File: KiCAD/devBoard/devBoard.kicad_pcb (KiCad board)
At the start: 2 copper layers, 31.1 x 66 mm, 4 parts, among them J1 Conn_02x14_Counter_Clockwise, J2 ISP_header_Conn_02x05_Odd_Even, J3 ISP_header_Conn_02x05_Odd_Even, J4 ISP_header_Conn_02x05_Odd_Even

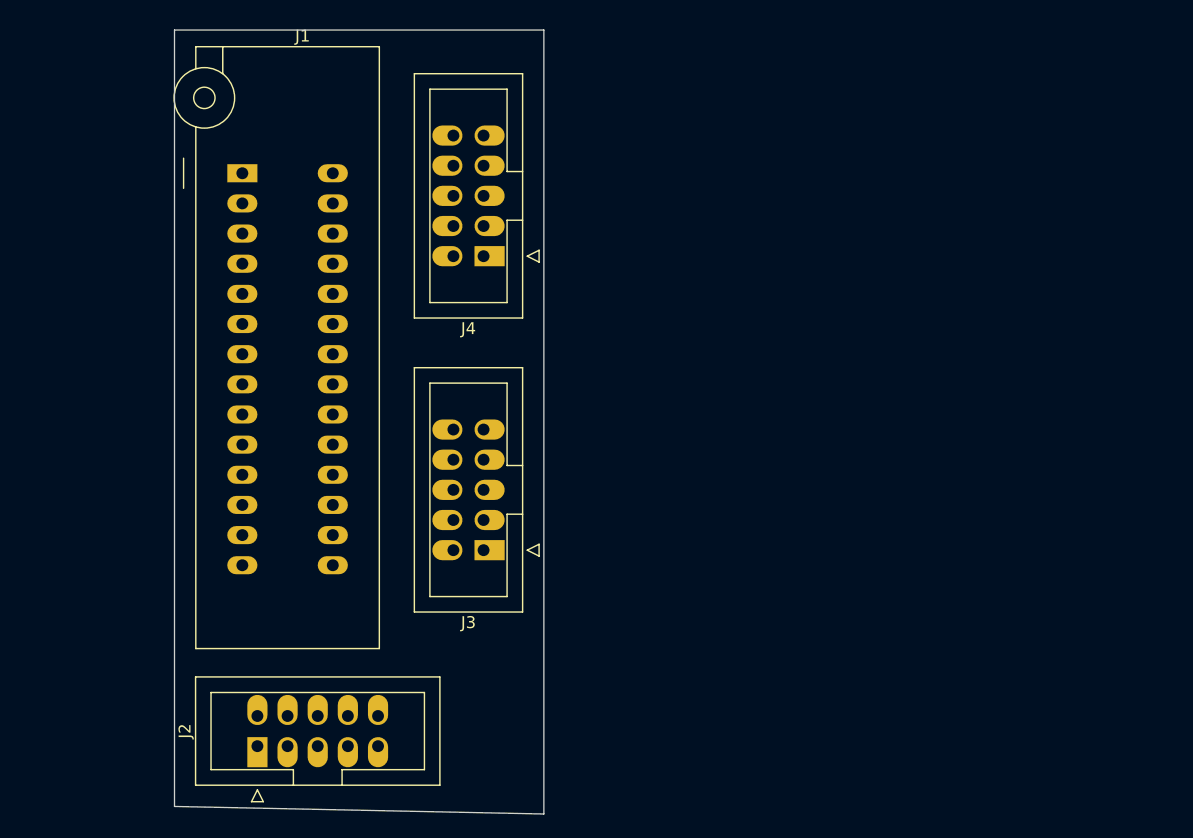
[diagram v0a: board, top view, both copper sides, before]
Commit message: devBoard, gerbers
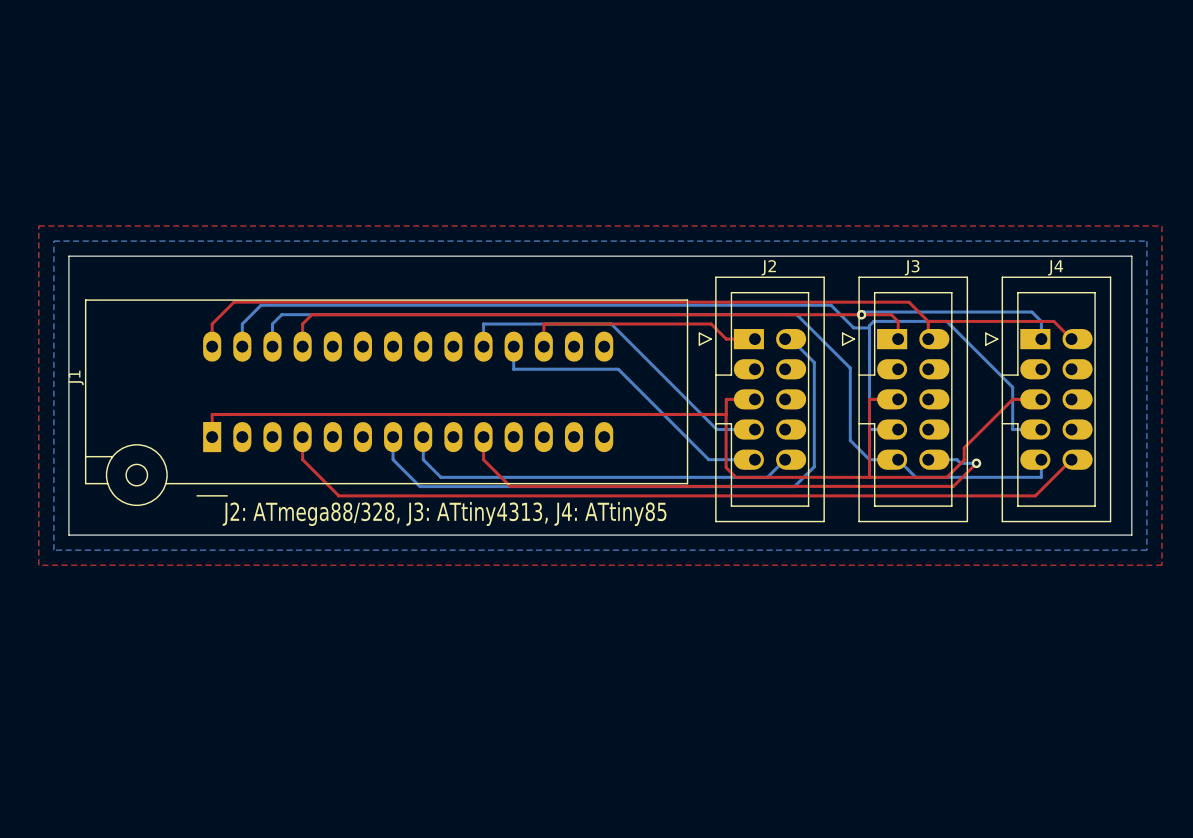
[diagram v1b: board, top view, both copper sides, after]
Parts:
- moved J2 54.2 mm to (188.6, 81.9), turned to 0 degrees
- moved J4 47.5 mm to (212.7, 81.9), turned to 0 degrees
- moved J3 39.2 mm to (200.7, 81.9), turned to 0 degrees
- moved J1 22.4 mm to (142.9, 90.2), turned to 90 degrees
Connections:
- J1 pad 20: 20 -> Net-(J1-Pad20)
- J1 pad 22: 22 -> Net-(J1-Pad22)
- J1 pad 7: 20 -> 7
- J1 pad 8: 22 -> 8
- J2 pad 10: 22 -> 8
- J2 pad 2: 20 -> 7
- J2 pad 8: 22 -> Net-(J2-Pad8)
- J3 pad 8: 10 -> Net-(J3-Pad8)
- J4 pad 8: 4 -> Net-(J4-Pad8)
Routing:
- net 1: track 0.00 -> 92.6 mm
- net 27: track 0.00 -> 87.8 mm
- net 28: track 0.00 -> 79.1 mm
- net 26: track 0.00 -> 77.7 mm
- net 25: track 0.00 -> 71.2 mm, vias 0 -> 1
- net 4: track 0.00 -> 69.2 mm
- net 7: track 0.00 -> 51.1 mm
- net 10: track 0.00 -> 49.3 mm, vias 0 -> 1
- net 8: track 0.00 -> 33.6 mm
- net 19: track 0.00 -> 28.4 mm
- net 18: track 0.00 -> 25.4 mm
- net 17: track 0.00 -> 20.2 mm
- added copper zone on B.Cu, net (none)
- added copper zone on F.Cu, net (none)
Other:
- board size 31.1 x 66 mm -> 89.5 x 23.5 mm
- board text added: "J2: ATmega88/328 J3: ATtiny4313 J4: ATtiny85"
- board text added: "J2: ATmega88/328, J3: ATtiny4313, J4: ATtiny85"
- board text added: "devBoard Design: Jon Sagebrand jonsagebrand@gmail.com"

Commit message: New PCBs
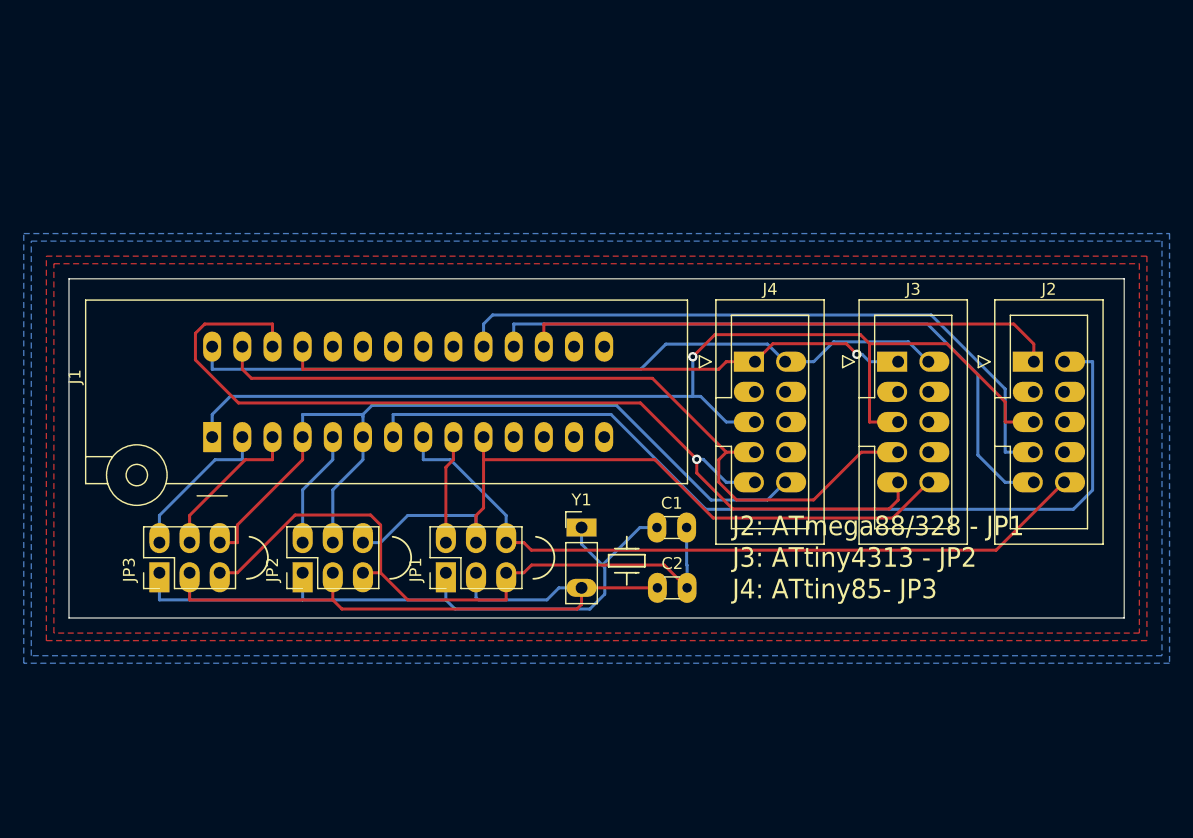
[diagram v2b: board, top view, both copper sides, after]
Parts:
- added C1: 22p, My_Misc:C_Disc_D3.0mm_W1.6mm_P2.50mm_larg, F.Cu at (180.3, 97.8)
- added C2: 22p, My_Misc:C_Disc_D3.0mm_W1.6mm_P2.50mm_larg, F.Cu at (180.4, 102.9)
- added JP1: 3_pole_Jumper_2_Open, My_Parts:3-pole_jumper_2x03_P2.54mm_Vertical, F.Cu at (162.6, 101.6)
- added JP2: 3_pole_Jumper_2_Open, My_Parts:3-pole_jumper_2x03_P2.54mm_Vertical, F.Cu at (150.5, 101.6)
- added JP3: 3_pole_Jumper_2_Open, My_Parts:3-pole_jumper_2x03_P2.54mm_Vertical, F.Cu at (138.4, 101.6)
- added Y1: Crystal, My_Headers:3-pin_Crystal_header_large, F.Cu at (174.0, 97.8)
- moved J4 24.2 mm to (188.6, 83.8)
- moved J2 23.6 mm to (212.1, 83.8)
- moved J3 1.90 mm to (200.7, 83.8)
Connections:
- J1 pad 2: Net-(J1-Pad2) -> 2
- J1 pad 3: Net-(J1-Pad3) -> 3
- J1 pad 5: Net-(J1-Pad5) -> 5
- J1 pad 6: Net-(J1-Pad6) -> 4
- J1 pad 9: Net-(J1-Pad9) -> 9
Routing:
- net XTAL1: track 0.00 -> 57.5 mm
- net XTAL2: track 0.00 -> 57.3 mm
- net GND: track 0.00 -> 56.6 mm
- net 18: track 25.4 -> 55.2 mm
- net 8: track 33.6 -> 62.7 mm
- net 19: track 28.4 -> 56.5 mm
- net 7: track 51.1 -> 78.0 mm
- net 17: track 20.2 -> 45.4 mm
- net 27: track 87.8 -> 68.2 mm
- net 25: track 71.2 -> 53.6 mm
- net 28: track 79.1 -> 65.1 mm
- net 10: track 49.3 -> 62.7 mm, vias 1 -> 0
- net 3: track 0.00 -> 13.1 mm
- net 2: track 0.00 -> 13.1 mm
- net 5: track 0.00 -> 9.94 mm
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- added copper zone on B.Cu, net GND
- added copper zone on F.Cu, net GND
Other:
- board size 89.5 x 23.5 mm -> 88.9 x 28.6 mm
- board text added: "J2: ATmega88/328 - JP1 J3: ATtiny4313 - JP2 J4: ATtiny85 - JP3"
- board text added: "J2: ATmega88/328 - JP1 J3: ATtiny4313 - JP2 J4: ATtiny85- JP3"
- board text removed: "J2: ATmega88/328 J3: ATtiny4313 J4: ATtiny85"
- board text removed: "J2: ATmega88/328, J3: ATtiny4313, J4: ATtiny85"

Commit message: kicad 6
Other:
- net class Default removed
